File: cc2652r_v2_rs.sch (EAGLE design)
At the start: 55 parts, among them IC3 CC2652R1FRGZ, SW1 MOMENTARY-SWITCH-SPST-SMD-4.6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, Y1 Q22FA12800150, Y2 32.768KHz

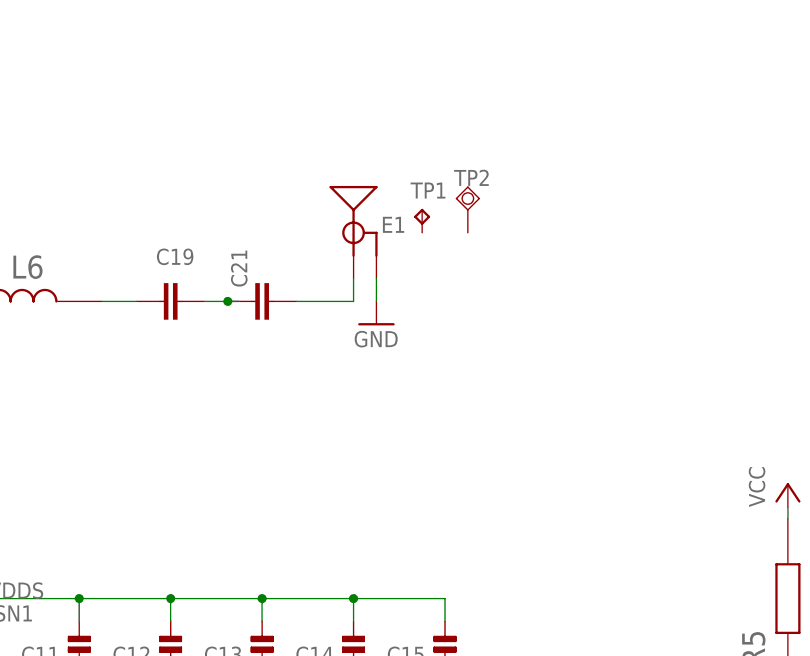
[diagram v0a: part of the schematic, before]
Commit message: Add files via upload
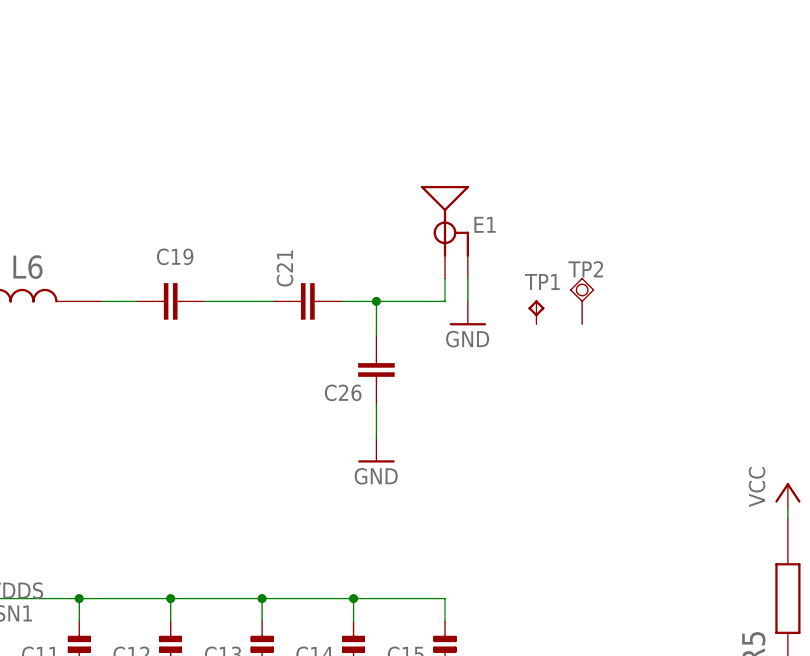
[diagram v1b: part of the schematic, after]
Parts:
- added C26: CAP0402, discretes-dev:CAP0402
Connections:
- net GND: now also C26.1
- net N$9: now also C26.2
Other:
- moved on the sheet: C21, E1, TP1, TP2
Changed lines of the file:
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@@
 <part name="P+9" library="supply1" library_urn="urn:adsk.eagle:library:371" deviceset="VCC" device=""/>
 <part name="P+10" library="supply1" library_urn="urn:adsk.eagle:library:371" deviceset="VCC" device=""/>
+<part name="C26" library="discretes-dev" deviceset="CAP0402" device=""/>
+<part name="GND31" library="supply1" library_urn="urn:adsk.eagle:library:371" deviceset="GND" device=""/>
 </parts>
 <sheets>
@@
 <attribute name="VALUE" x="106.68" y="5.08" size="1.778" layer="96"/>
 </instance>
-<instance part="E1" gate="G$1" x="203.2" y="104.14" smashed="yes">
-<attribute name="NAME" x="206.248" y="99.06" size="1.778" layer="95" font="vector"/>
-</instance>
-<instance part="C21" gate="G$1" x="193.04" y="91.44" smashed="yes" rot="R90">
-<attribute name="NAME" x="191.389" y="92.964" size="1.778" layer="95" font="vector" rot="R90"/>
-</instance>
-<instance part="GND7" gate="1" x="205.74" y="88.9" smashed="yes">
-<attribute name="VALUE" x="203.2" y="86.36" size="1.778" layer="96"/>
-</instance>
-<instance part="TP1" gate="G$1" x="210.82" y="101.6" smashed="yes">
-<attribute name="NAME" x="209.55" y="102.87" size="1.778" layer="95"/>
-<attribute name="TP_SIGNAL_NAME" x="212.09" y="100.33" size="1.778" layer="97"/>
-</instance>
-<instance part="TP2" gate="G$1" x="215.9" y="101.6" smashed="yes" rot="R180">
-<attribute name="NAME" x="218.44" y="106.045" size="1.778" layer="95" rot="R180"/>
-<attribute name="TP_SIGNAL_NAME" x="213.36" y="102.87" size="1.778" layer="97" rot="R180"/>
+<instance part="E1" gate="G$1" x="213.36" y="104.14" smashed="yes">
+<attribute name="NAME" x="216.408" y="99.06" size="1.778" layer="95" font="vector"/>
+</instance>
+<instance part="C21" gate="G$1" x="198.12" y="91.44" smashed="yes" rot="R90">
+<attribute name="NAME" x="196.469" y="92.964" size="1.778" layer="95" font="vector" rot="R90"/>
+</instance>
+<instance part="GND7" gate="1" x="215.9" y="88.9" smashed="yes">
+<attribute name="VALUE" x="213.36" y="86.36" size="1.778" layer="96"/>
+</instance>
+<instance part="TP1" gate="G$1" x="223.52" y="91.44" smashed="yes">
+<attribute name="NAME" x="222.25" y="92.71" size="1.778" layer="95"/>
+<attribute name="TP_SIGNAL_NAME" x="224.79" y="90.17" size="1.778" layer="97"/>
+</instance>
+<instance part="TP2" gate="G$1" x="228.6" y="91.44" smashed="yes" rot="R180">
+<attribute name="NAME" x="231.14" y="95.885" size="1.778" layer="95" rot="R180"/>
+<attribute name="TP_SIGNAL_NAME" x="226.06" y="92.71" size="1.778" layer="97" rot="R180"/>
 </instance>
 <instance part="BT1" gate="G$1" x="157.48" y="43.18" smashed="yes">
@@
 <instance part="P+10" gate="VCC" x="259.08" y="71.12" smashed="yes">
 <attribute name="VALUE" x="256.54" y="68.58" size="1.778" layer="96" rot="R90"/>
+</instance>
+<instance part="C26" gate="G$1" x="205.74" y="83.82" smashed="yes" rot="R180">
+<attribute name="NAME" x="204.216" y="82.169" size="1.778" layer="95" font="vector" rot="R180"/>
+</instance>
+<instance part="GND31" gate="1" x="205.74" y="73.66" smashed="yes">
+<attribute name="VALUE" x="203.2" y="71.12" size="1.778" layer="96"/>
 </instance>
 </instances>
@@
 <segment>
 <pinref part="E1" gate="G$1" pin="GND"/>
-<wire x1="205.74" y1="93.98" x2="205.74" y2="91.44" width="0.1524" layer="91"/>
+<wire x1="215.9" y1="93.98" x2="215.9" y2="91.44" width="0.1524" layer="91"/>
 <pinref part="GND7" gate="1" pin="GND"/>
 </segment>
@@
 <wire x1="119.38" y1="10.16" x2="119.38" y2="11.43" width="0.1524" layer="91"/>
 <pinref part="R3" gate="G$1" pin="1"/>
+</segment>
+<segment>
+<pinref part="C26" gate="G$1" pin="1"/>
+<pinref part="GND31" gate="1" pin="GND"/>
+<wire x1="205.74" y1="80.01" x2="205.74" y2="76.2" width="0.1524" layer="91"/>
 </segment>
 </net>
@@
 </segment>
 </net>
-<net name="N$8" class="0">
-<segment>
-<pinref part="C19" gate="G$1" pin="2"/>
-<wire x1="190.5" y1="91.44" x2="189.23" y2="91.44" width="0.1524" layer="91"/>
-<pinref part="C21" gate="G$1" pin="1"/>
-<wire x1="189.23" y1="91.44" x2="186.69" y2="91.44" width="0.1524" layer="91"/>
-<junction x="189.23" y="91.44"/>
-</segment>
-</net>
 <net name="N$10" class="0">
 <segment>
@@
 <segment>
 <pinref part="C21" gate="G$1" pin="2"/>
-<wire x1="196.85" y1="91.44" x2="203.2" y2="91.44" width="0.1524" layer="91"/>
+<wire x1="201.93" y1="91.44" x2="205.74" y2="91.44" width="0.1524" layer="91"/>
 <pinref part="E1" gate="G$1" pin="SIGNAL"/>
-<wire x1="203.2" y1="91.44" x2="203.2" y2="93.98" width="0.1524" layer="91"/>
-</segment>
-</net>
+<wire x1="205.74" y1="91.44" x2="213.36" y2="91.44" width="0.1524" layer="91"/>
+<wire x1="213.36" y1="91.44" x2="213.36" y2="93.98" width="0.1524" layer="91"/>
+<pinref part="C26" gate="G$1" pin="2"/>
+<wire x1="205.74" y1="91.44" x2="205.74" y2="87.63" width="0.1524" layer="91"/>
+<junction x="205.74" y="91.44"/>
+</segment>
+</net>
+<net name="N$7" class="0">
+<segment>
+<pinref part="C19" gate="G$1" pin="2"/>
+<pinref part="C21" gate="G$1" pin="1"/>
+<wire x1="186.69" y1="91.44" x2="194.31" y2="91.44" width="0.1524" layer="91"/>
+</segment>
+</net>
